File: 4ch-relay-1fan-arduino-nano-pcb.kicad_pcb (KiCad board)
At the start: 2 copper layers, 62 parts, among them J1 Screw_Terminal_01x03, J2 Conn_01x08_Pin, J3 Screw_Terminal_01x03, J4 Screw_Terminal_01x03, J5 Screw_Terminal_01x03, J7 Conn_01x07_Pin, J9 Conn_01x04_Pin, K1 Relay_SPDT, K2 Relay_SPDT, K3 Relay_SPDT, K4 Relay_SPDT, Q1 2N3904, Q2 2N3904, Q3 2N3904, Q4 2N3904, Q5 BT136, U1 PC817, U2 PC817, U3 PC817, U4 PC817, U5 MOC3021M, U6 PC817, U7 TSOP1738, U8 HLK-10M05

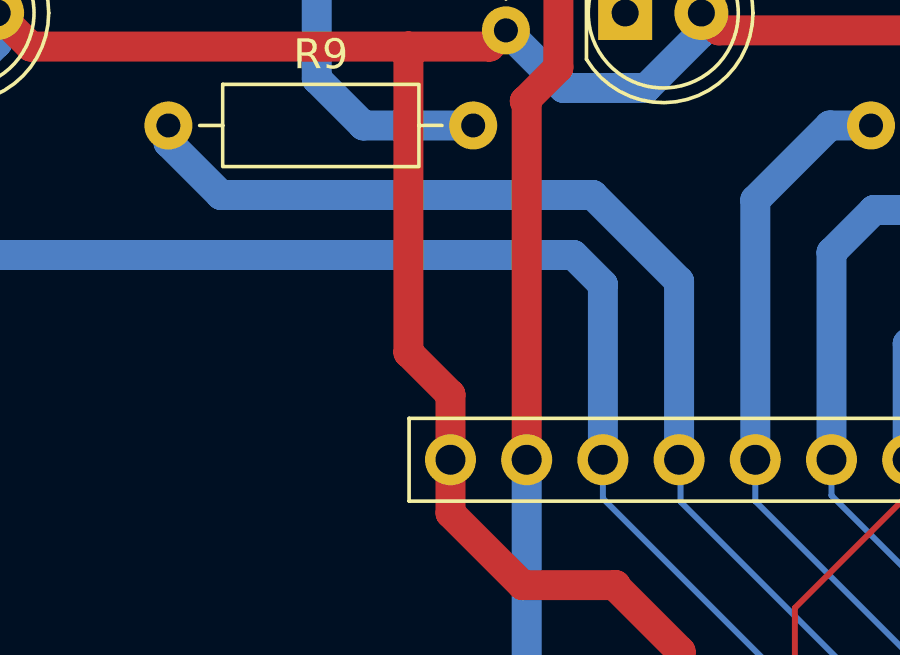
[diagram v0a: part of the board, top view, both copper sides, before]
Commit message: Add files via upload
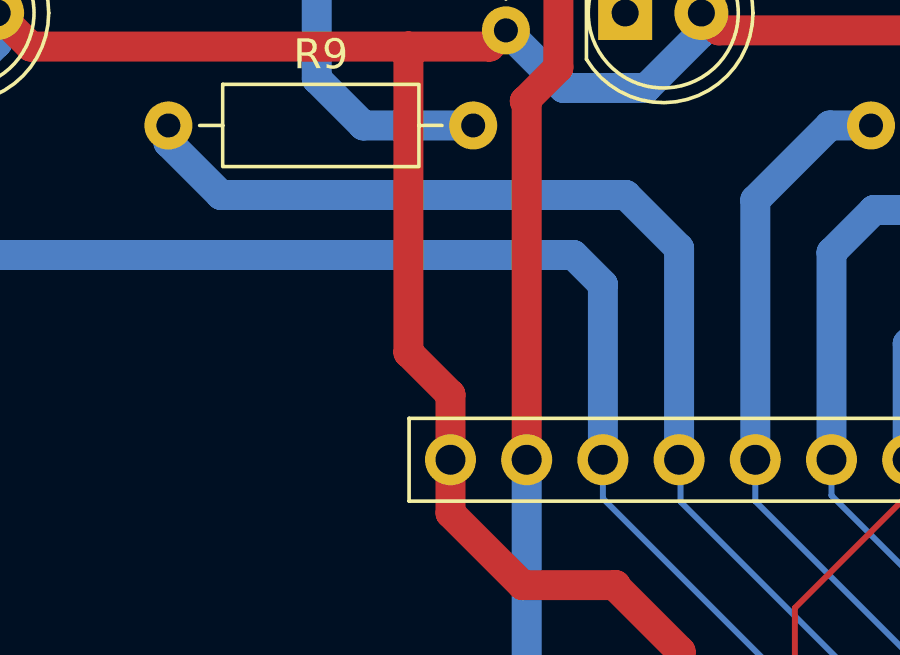
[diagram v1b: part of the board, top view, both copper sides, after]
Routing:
- net Net-(A1-D6): track 54.8 -> 55.5 mm
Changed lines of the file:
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@@
 	)
 	(segment
-		(start 123.7725 102.2025)
-		(end 123.7725 108.1525)
+		(start 108.5 99.3275)
+		(end 121.9975 99.3275)
+		(width 1)
+		(layer "B.Cu")
+		(net "Net-(A1-D6)")
+	)
+	(segment
+		(start 121.9975 99.3275)
+		(end 123.7725 101.1025)
 		(width 1)
 		(layer "B.Cu")
@@
 	)
 	(segment
-		(start 120.8975 99.3275)
-		(end 123.7725 102.2025)
+		(start 106.75 97.5775)
+		(end 108.5 99.3275)
 		(width 1)
 		(layer "B.Cu")
@@
 	)
 	(segment
-		(start 108.5 99.3275)
-		(end 120.8975 99.3275)
+		(start 123.7725 101.1025)
+		(end 123.7725 108.1525)
 		(width 1)
 		(layer "B.Cu")
@@
 		(layer "B.Cu")
 		(net "Net-(A1-D6)")
-	)
-	(segment
-		(start 106.75 97.5775)
-		(end 108.5 99.3275)
-		(width 1)
-		(layer "B.Cu")
-		(net "Net-(A1-D6)")
